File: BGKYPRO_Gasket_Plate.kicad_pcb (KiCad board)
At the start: 2 copper layers, 294 x 104 mm, 0 parts

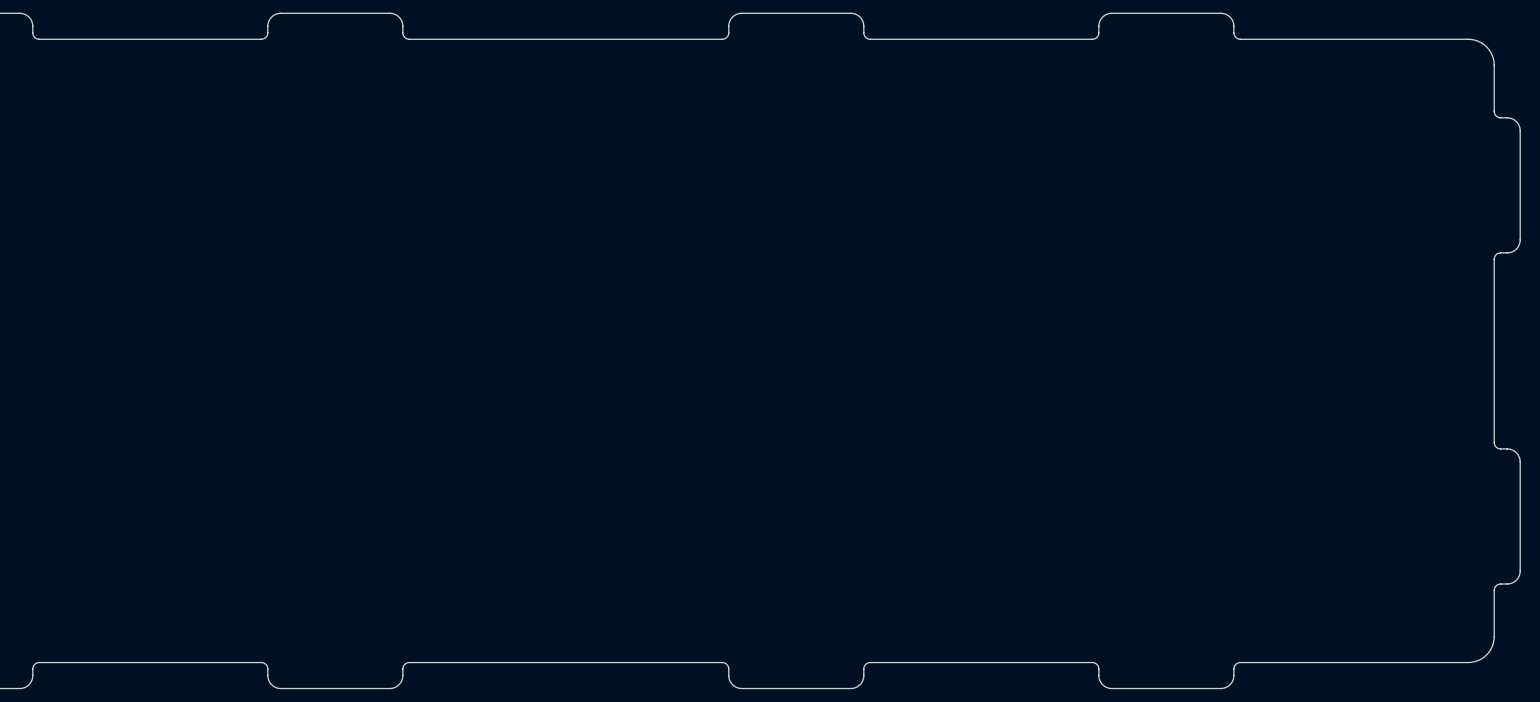
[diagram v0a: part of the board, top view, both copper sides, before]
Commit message: fix
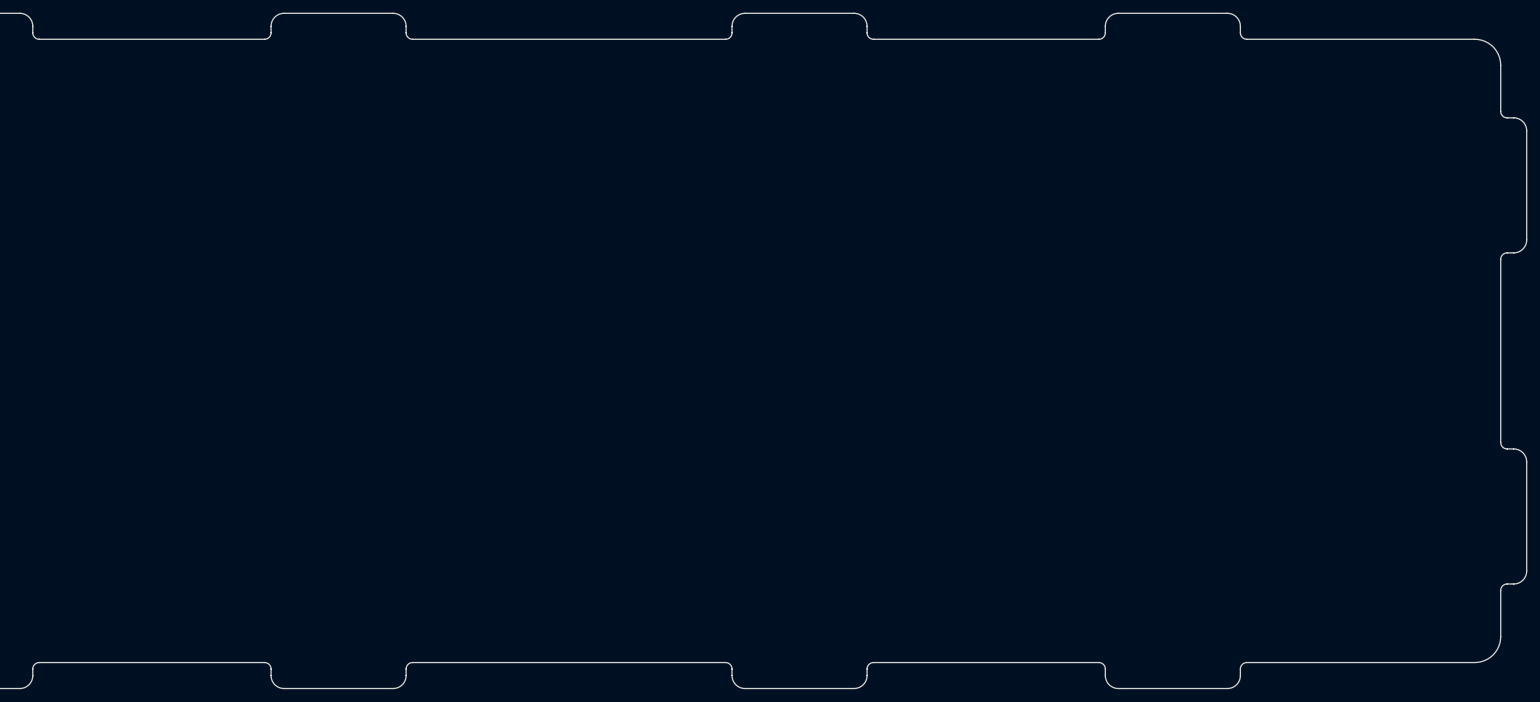
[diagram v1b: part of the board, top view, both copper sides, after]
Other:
- board size 294 x 104 mm -> 295 x 104 mm
